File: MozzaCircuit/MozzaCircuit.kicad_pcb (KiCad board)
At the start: 2 copper layers, 11 parts

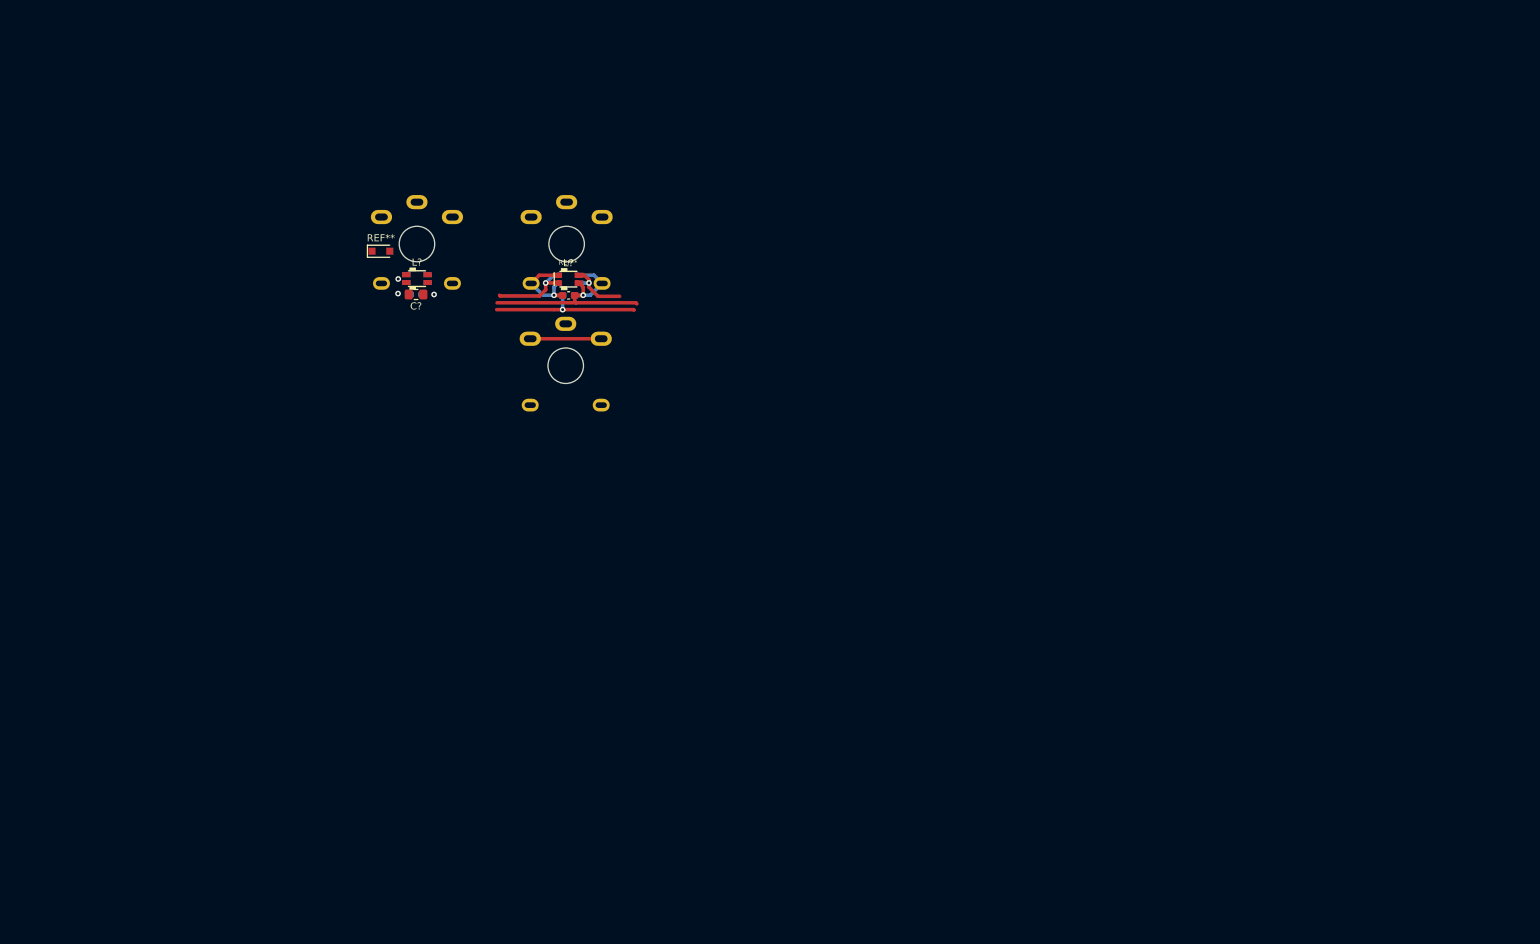
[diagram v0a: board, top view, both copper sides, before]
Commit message: init pcb
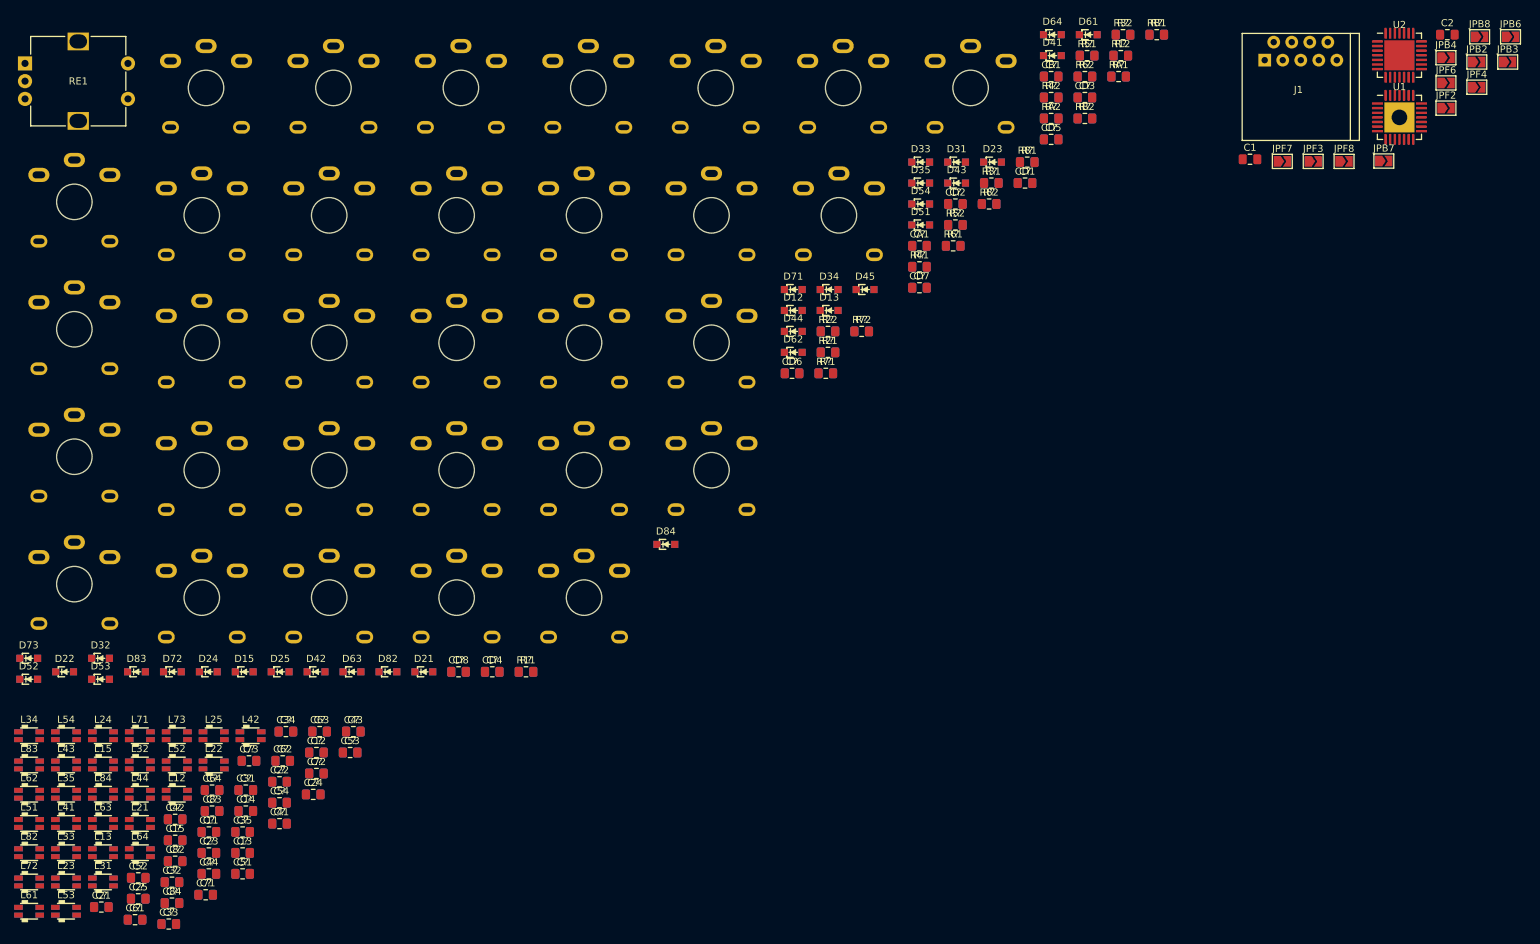
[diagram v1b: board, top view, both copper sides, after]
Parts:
- removed C?: C_2012, 00_KeyParts:C_2012
- removed L? (x2): WS2812B, 00_KeyParts:WS2812B_2020_rev
- removed REF** (x3): ChocV2_rev, 00_KeyParts:ChocV2_rev
- removed REF** (x3): C_0603_1608Metric_Pad1.08x0.95mm_HandSolder, Capacitor_SMD:C_0603_1608Metric_Pad1.08x0.95mm_HandSolder
- removed REF**: D_SOD-323_HandSoldering, Diode_SMD:D_SOD-323_HandSoldering
- removed REF**: WS2812C-2020, 00_KeyParts:LED_WS2812C-2020_BackMount_v2
- added C1: 0.1u, 00_KeyParts:C_2012, F.Cu at (206.2, 46.5)
- added C11: 0.1u, 00_KeyParts:C_2012_rev, F.Cu at (59.6, 141.2)
- added C12: C_Small, 00_KeyParts:C_2012_rev, F.Cu at (74.7, 130.1)
- added C13: C_Small, 00_KeyParts:C_2012_rev, F.Cu at (64.3, 144.2)
- added C14: C_Small, 00_KeyParts:C_2012_rev, F.Cu at (64.8, 138.3)
- added C15: C_Small, 00_KeyParts:C_2012_rev, F.Cu at (54.8, 142.4)
- added C2: C_Small, 00_KeyParts:C_2012, F.Cu at (234.0, 28.9)
- added C21: C_Small, 00_KeyParts:C_2012_rev, F.Cu at (44.4, 151.8)
- added C22: C_Small, 00_KeyParts:C_2012_rev, F.Cu at (69.5, 134.2)
- added C23: C_Small, 00_KeyParts:C_2012_rev, F.Cu at (59.6, 144.2)
- added C24: C_Small, 00_KeyParts:C_2012_rev, F.Cu at (74.3, 136.0)
- added C25: C_Small, 00_KeyParts:C_2012_rev, F.Cu at (49.6, 150.7)
- added C31: C_Small, 00_KeyParts:C_2012_rev, F.Cu at (64.8, 135.3)
- added C32: C_Small, 00_KeyParts:C_2012_rev, F.Cu at (54.4, 148.3)
- added C33: C_Small, 00_KeyParts:C_2012_rev, F.Cu at (53.9, 154.2)
- added C34: C_Small, 00_KeyParts:C_2012_rev, F.Cu at (70.4, 127.1)
- added C35: C_Small, 00_KeyParts:C_2012_rev, F.Cu at (64.3, 141.2)
- added C41: C_Small, 00_KeyParts:C_2012_rev, F.Cu at (69.5, 140.1)
- added C42: C_Small, 00_KeyParts:C_2012_rev, F.Cu at (54.8, 139.5)
- added C43: C_Small, 00_KeyParts:C_2012_rev, F.Cu at (79.9, 127.1)
- added C44: C_Small, 00_KeyParts:C_2012_rev, F.Cu at (59.6, 147.1)
- added C51: C_Small, 00_KeyParts:C_2012_rev, F.Cu at (64.3, 147.1)
- added C52: C_Small, 00_KeyParts:C_2012_rev, F.Cu at (49.6, 147.7)
- added C53: C_Small, 00_KeyParts:C_2012_rev, F.Cu at (79.5, 130.1)
- added C54: C_Small, 00_KeyParts:C_2012_rev, F.Cu at (69.5, 137.1)
- added C61: C_Small, 00_KeyParts:C_2012_rev, F.Cu at (49.2, 153.6)
- added C62: C_Small, 00_KeyParts:C_2012_rev, F.Cu at (70.0, 131.2)
- added C63: C_Small, 00_KeyParts:C_2012_rev, F.Cu at (75.2, 127.1)
- added C64: C_Small, 00_KeyParts:C_2012_rev, F.Cu at (60.0, 135.3)
- added C71: C_Small, 00_KeyParts:C_2012_rev, F.Cu at (59.1, 150.1)
- added C72: C_Small, 00_KeyParts:C_2012_rev, F.Cu at (74.7, 133.0)
- added C73: C_Small, 00_KeyParts:C_2012_rev, F.Cu at (65.2, 131.2)
- added C82: C_Small, 00_KeyParts:C_2012_rev, F.Cu at (54.8, 145.4)
- added C83: C_Small, 00_KeyParts:C_2012_rev, F.Cu at (60.0, 138.3)
- added C84: C_Small, 00_KeyParts:C_2012_rev, F.Cu at (54.4, 151.3)
- added CA1: 33n, 00_KeyParts:C_2012_rev, F.Cu at (159.7, 58.7)
- added CB1: C_Small, 00_KeyParts:C_2012_rev, F.Cu at (178.2, 34.8)
- added CD1: 33n, 00_KeyParts:C_2012_rev, F.Cu at (174.6, 49.8)
- added CD2: C_Small, 00_KeyParts:C_2012_rev, F.Cu at (164.7, 52.8)
- added CD3: C_Small, 00_KeyParts:C_2012_rev, F.Cu at (183.0, 37.8)
- added CD4: C_Small, 00_KeyParts:C_2012_rev, F.Cu at (99.5, 118.7)
- added CD5: C_Small, 00_KeyParts:C_2012_rev, F.Cu at (178.2, 43.7)
- added CD6: C_Small, 00_KeyParts:C_2012_rev, F.Cu at (141.7, 76.6)
- added CD7: C_Small, 00_KeyParts:C_2012_rev, F.Cu at (159.7, 64.6)
- added CD8: C_Small, 00_KeyParts:C_2012_rev, F.Cu at (94.8, 118.7)
- added D12: D_Small, 00_KeyParts:D_SOD-323_both_sides, F.Cu at (141.9, 67.8)
- added D13: D_Small, 00_KeyParts:D_SOD-323_both_sides, F.Cu at (147.0, 67.8)
- added D15: D_Small, 00_KeyParts:D_SOD-323_both_sides, F.Cu at (64.6, 118.7)
- added D21: D_Small, 00_KeyParts:D_SOD-323_both_sides, F.Cu at (89.9, 118.7)
- added D22: D_Small, 00_KeyParts:D_SOD-323_both_sides, F.Cu at (39.3, 118.7)
- added D23: D_Small, 00_KeyParts:D_SOD-323_both_sides, F.Cu at (170.0, 46.9)
- added D24: D_Small, 00_KeyParts:D_SOD-323_both_sides, F.Cu at (59.5, 118.7)
- added D25: D_Small, 00_KeyParts:D_SOD-323_both_sides, F.Cu at (69.6, 118.7)
- added D31: D_Small, 00_KeyParts:D_SOD-323_both_sides, F.Cu at (164.9, 46.9)
- added D32: D_Small, 00_KeyParts:D_SOD-323_both_sides, F.Cu at (44.3, 116.8)
- added D33: D_Small, 00_KeyParts:D_SOD-323_both_sides, F.Cu at (159.9, 46.9)
- added D34: D_Small, 00_KeyParts:D_SOD-323_both_sides, F.Cu at (147.0, 64.8)
- added D35: D_Small, 00_KeyParts:D_SOD-323_both_sides, F.Cu at (159.9, 49.8)
- added D41: D_Small, 00_KeyParts:D_SOD-323_both_sides, F.Cu at (178.4, 31.9)
- added D42: D_Small, 00_KeyParts:D_SOD-323_both_sides, F.Cu at (74.7, 118.7)
- added D43: D_Small, 00_KeyParts:D_SOD-323_both_sides, F.Cu at (164.9, 49.8)
- added D44: D_Small, 00_KeyParts:D_SOD-323_both_sides, F.Cu at (141.9, 70.7)
- added D45: D_Small, 00_KeyParts:D_SOD-323_both_sides, F.Cu at (152.0, 64.8)
- added D51: D_Small, 00_KeyParts:D_SOD-323_both_sides, F.Cu at (159.9, 55.7)
- added D52: D_Small, 00_KeyParts:D_SOD-323_both_sides, F.Cu at (34.2, 119.7)
- added D53: D_Small, 00_KeyParts:D_SOD-323_both_sides, F.Cu at (44.3, 119.7)
- added D54: D_Small, 00_KeyParts:D_SOD-323_both_sides, F.Cu at (159.9, 52.8)
- added D61: D_Small, 00_KeyParts:D_SOD-323_both_sides, F.Cu at (183.5, 28.9)
- added D62: D_Small, 00_KeyParts:D_SOD-323_both_sides, F.Cu at (141.9, 73.7)
- added D63: D_Small, 00_KeyParts:D_SOD-323_both_sides, F.Cu at (79.7, 118.7)
- added D64: D_Small, 00_KeyParts:D_SOD-323_both_sides, F.Cu at (178.4, 28.9)
- added D71: D_Small, 00_KeyParts:D_SOD-323_both_sides, F.Cu at (141.9, 64.8)
- added D72: D_Small, 00_KeyParts:D_SOD-323_both_sides, F.Cu at (54.4, 118.7)
- added D73: D_Small, 00_KeyParts:D_SOD-323_both_sides, F.Cu at (34.2, 116.8)
- added D82: D_Small, 00_KeyParts:D_SOD-323_both_sides, F.Cu at (84.8, 118.7)
- added D83: D_Small, 00_KeyParts:D_SOD-323_both_sides, F.Cu at (49.4, 118.7)
- added D84: D_Small, 00_KeyParts:D_SOD-323_both_sides, F.Cu at (124.0, 100.7)
- added J1: 8P8C_both_sides, 00_KeyParts:RJ45_Molex_0955032884_both_sides, F.Cu at (213.4, 30.0)
- added JPB2: SolderJumper_2_Open, Jumper:SolderJumper-2_P1.3mm_Open_TrianglePad1.0x1.5mm, F.Cu at (238.2, 32.8)
- added JPB3: SolderJumper_2_Open, Jumper:SolderJumper-2_P1.3mm_Open_TrianglePad1.0x1.5mm, F.Cu at (242.5, 32.8)
- added JPB4: SolderJumper_2_Open, Jumper:SolderJumper-2_P1.3mm_Open_TrianglePad1.0x1.5mm, F.Cu at (233.8, 32.2)
- added JPB6: SolderJumper_2_Open, Jumper:SolderJumper-2_P1.3mm_Open_TrianglePad1.0x1.5mm, F.Cu at (242.9, 29.2)
- added JPB7: SolderJumper_2_Open, Jumper:SolderJumper-2_P1.3mm_Open_TrianglePad1.0x1.5mm, F.Cu at (225.1, 46.7)
- added JPB8: SolderJumper_2_Open, Jumper:SolderJumper-2_P1.3mm_Open_TrianglePad1.0x1.5mm, F.Cu at (238.6, 29.2)
- added JPF2: SolderJumper_2_Open, Jumper:SolderJumper-2_P1.3mm_Open_TrianglePad1.0x1.5mm, F.Cu at (233.8, 39.3)
- added JPF3: SolderJumper_2_Open, Jumper:SolderJumper-2_P1.3mm_Open_TrianglePad1.0x1.5mm, F.Cu at (215.1, 46.8)
- added JPF4: SolderJumper_2_Open, Jumper:SolderJumper-2_P1.3mm_Open_TrianglePad1.0x1.5mm, F.Cu at (238.2, 36.3)
- added JPF6: SolderJumper_2_Open, Jumper:SolderJumper-2_P1.3mm_Open_TrianglePad1.0x1.5mm, F.Cu at (233.8, 35.7)
- added JPF7: SolderJumper_2_Open, Jumper:SolderJumper-2_P1.3mm_Open_TrianglePad1.0x1.5mm, F.Cu at (210.8, 46.8)
- added JPF8: SolderJumper_2_Open, Jumper:SolderJumper-2_P1.3mm_Open_TrianglePad1.0x1.5mm, F.Cu at (219.5, 46.8)
- added L12: WS2812-2020_both_sides, 00_KeyParts:WS2812B_2020_rev, F.Cu at (55.1, 135.9)
- added L13: WS2812-2020_both_sides, 00_KeyParts:WS2812B_2020_rev, F.Cu at (44.7, 144.2)
- added L15: WS2812-2020_both_sides, 00_KeyParts:WS2812B_2020_rev, F.Cu at (44.7, 131.8)
- added L21: WS2812-2020_both_sides, 00_KeyParts:WS2812B_2020_rev, F.Cu at (49.9, 140.0)
- added L22: WS2812-2020_both_sides, 00_KeyParts:WS2812B_2020_rev, F.Cu at (60.3, 131.8)
- added L23: WS2812-2020_both_sides, 00_KeyParts:WS2812B_2020_rev, F.Cu at (39.5, 148.3)
- added L24: WS2812-2020_both_sides, 00_KeyParts:WS2812B_2020_rev, F.Cu at (44.7, 127.7)
- added L25: WS2812-2020_both_sides, 00_KeyParts:WS2812B_2020_rev, F.Cu at (60.3, 127.7)
- added L31: WS2812-2020_both_sides, 00_KeyParts:WS2812B_2020_rev, F.Cu at (44.7, 148.3)
- added L32: WS2812-2020_both_sides, 00_KeyParts:WS2812B_2020_rev, F.Cu at (49.9, 131.8)
- added L33: WS2812-2020_both_sides, 00_KeyParts:WS2812B_2020_rev, F.Cu at (39.5, 144.2)
- added L34: WS2812-2020_both_sides, 00_KeyParts:WS2812B_2020_rev, F.Cu at (34.3, 127.7)
- added L35: WS2812-2020_both_sides, 00_KeyParts:WS2812B_2020_rev, F.Cu at (39.5, 135.9)
- added L41: WS2812-2020_both_sides, 00_KeyParts:WS2812B_2020_rev, F.Cu at (39.5, 140.0)
- added L42: WS2812-2020_both_sides, 00_KeyParts:WS2812B_2020_rev, F.Cu at (65.5, 127.7)
- added L43: WS2812-2020_both_sides, 00_KeyParts:WS2812B_2020_rev, F.Cu at (39.5, 131.8)
- added L44: WS2812-2020_both_sides, 00_KeyParts:WS2812B_2020_rev, F.Cu at (49.9, 135.9)
- added L51: WS2812-2020_both_sides, 00_KeyParts:WS2812B_2020_rev, F.Cu at (34.3, 140.0)
- added L52: WS2812-2020_both_sides, 00_KeyParts:WS2812B_2020_rev, F.Cu at (55.1, 131.8)
- added L53: WS2812-2020_both_sides, 00_KeyParts:WS2812B_2020_rev, F.Cu at (39.5, 152.4)
- added L54: WS2812-2020_both_sides, 00_KeyParts:WS2812B_2020_rev, F.Cu at (39.5, 127.7)
- added L61: WS2812-2020_both_sides, 00_KeyParts:WS2812B_2020_rev, F.Cu at (34.3, 152.4)
- added L62: WS2812-2020_both_sides, 00_KeyParts:WS2812B_2020_rev, F.Cu at (34.3, 135.9)
- added L63: WS2812-2020_both_sides, 00_KeyParts:WS2812B_2020_rev, F.Cu at (44.7, 140.0)
- added L64: WS2812-2020_both_sides, 00_KeyParts:WS2812B_2020_rev, F.Cu at (49.9, 144.2)
- added L71: WS2812-2020_both_sides, 00_KeyParts:WS2812B_2020_rev, F.Cu at (49.9, 127.7)
- added L72: WS2812-2020_both_sides, 00_KeyParts:WS2812B_2020_rev, F.Cu at (34.3, 148.3)
- added L73: WS2812-2020_both_sides, 00_KeyParts:WS2812B_2020_rev, F.Cu at (55.1, 127.7)
- added L82: WS2812-2020_both_sides, 00_KeyParts:WS2812B_2020_rev, F.Cu at (34.3, 144.2)
- added L83: WS2812-2020_both_sides, 00_KeyParts:WS2812B_2020_rev, F.Cu at (34.3, 131.8)
- added L84: WS2812-2020_both_sides, 00_KeyParts:WS2812B_2020_rev, F.Cu at (44.7, 135.9)
- added R11: 10k, 00_KeyParts:R_2012_rev, F.Cu at (104.3, 118.7)
- added R12: 4k7, 00_KeyParts:R_2012_rev, F.Cu at (188.0, 31.9)
- added R21: R_Small_US, 00_KeyParts:R_2012_rev, F.Cu at (146.8, 73.7)
- added R22: R_Small_US, 00_KeyParts:R_2012_rev, F.Cu at (146.8, 70.7)
- added R31: R_Small_US, 00_KeyParts:R_2012_rev, F.Cu at (169.8, 49.8)
- added R32: R_Small_US, 00_KeyParts:R_2012_rev, F.Cu at (188.4, 28.9)
- added R41: R_Small_US, 00_KeyParts:R_2012_rev, F.Cu at (159.7, 61.6)
- added R42: R_Small_US, 00_KeyParts:R_2012_rev, F.Cu at (178.2, 37.8)
- added R51: R_Small_US, 00_KeyParts:R_2012_rev, F.Cu at (183.3, 31.9)
- added R52: R_Small_US, 00_KeyParts:R_2012_rev, F.Cu at (164.7, 55.7)
- added R61: R_Small_US, 00_KeyParts:R_2012_rev, F.Cu at (164.4, 58.7)
- added R62: R_Small_US, 00_KeyParts:R_2012_rev, F.Cu at (183.0, 34.8)
- added R71: R_Small_US, 00_KeyParts:R_2012_rev, F.Cu at (146.5, 76.6)
- added R72: R_Small_US, 00_KeyParts:R_2012_rev, F.Cu at (151.5, 70.7)
- added R81: R_Small_US, 00_KeyParts:R_2012_rev, F.Cu at (174.9, 46.9)
- added R82: R_Small_US, 00_KeyParts:R_2012_rev, F.Cu at (169.5, 52.8)
- added RA1: 10k, 00_KeyParts:R_2012_rev, F.Cu at (187.7, 34.8)
- added RA2: 4k7, 00_KeyParts:R_2012_rev, F.Cu at (178.2, 40.7)
- added RB1: R_Small_US, 00_KeyParts:R_2012_rev, F.Cu at (193.1, 28.9)
- added RB2: R_Small_US, 00_KeyParts:R_2012_rev, F.Cu at (183.0, 40.7)
- added RE1: RotaryEncoder_Switch, 00_KeyParts:RotaryEncoder_Bourns_PEC12R-4215F, F.Cu at (41.2, 35.5)
- added SW12: SW_ChocV2_rev, 00_KeyParts:ChocV2_rev, F.Cu at (113.0, 36.4)
- added SW13: SW_ChocV2_rev, 00_KeyParts:ChocV2_rev, F.Cu at (76.5, 108.2)
- added SW15: SW_ChocV2_rev, 00_KeyParts:ChocV2_rev, F.Cu at (40.6, 106.3)
- added SW21: SW_ChocV2_rev, 00_KeyParts:ChocV2_rev, F.Cu at (58.6, 72.3)
- added SW22: SW_ChocV2_rev, 00_KeyParts:ChocV2_rev, F.Cu at (59.2, 36.4)
- added SW23: SW_ChocV2_rev, 00_KeyParts:ChocV2_rev, F.Cu at (130.4, 72.3)
- added SW24: SW_ChocV2_rev, 00_KeyParts:ChocV2_rev, F.Cu at (40.6, 52.5)
- added SW25: SW_ChocV2_rev, 00_KeyParts:ChocV2_rev, F.Cu at (77.1, 36.4)
- added SW31: SW_ChocV2_rev, 00_KeyParts:ChocV2_rev, F.Cu at (148.9, 36.4)
- added SW32: SW_ChocV2_rev, 00_KeyParts:ChocV2_rev, F.Cu at (112.4, 72.3)
- added SW33: SW_ChocV2_rev, 00_KeyParts:ChocV2_rev, F.Cu at (76.5, 90.3)
- added SW34: SW_ChocV2_rev, 00_KeyParts:ChocV2_rev, F.Cu at (112.4, 54.4)
- added SW35: SW_ChocV2_rev, 00_KeyParts:ChocV2_rev, F.Cu at (94.5, 72.3)
- added SW41: SW_ChocV2_rev, 00_KeyParts:ChocV2_rev, F.Cu at (166.9, 36.4)
- added SW42: SW_ChocV2_rev, 00_KeyParts:ChocV2_rev, F.Cu at (40.6, 70.4)
- added SW43: SW_ChocV2_rev, 00_KeyParts:ChocV2_rev, F.Cu at (130.4, 90.3)
- added SW44: SW_ChocV2_rev, 00_KeyParts:ChocV2_rev, F.Cu at (94.5, 90.3)
- added SW51: SW_ChocV2_rev, 00_KeyParts:ChocV2_rev, F.Cu at (76.5, 54.4)
- added SW52: SW_ChocV2_rev, 00_KeyParts:ChocV2_rev, F.Cu at (131.0, 36.4)
- added SW53: SW_ChocV2_rev, 00_KeyParts:ChocV2_rev, F.Cu at (130.4, 54.4)
- added SW54: SW_ChocV2_rev, 00_KeyParts:ChocV2_rev, F.Cu at (94.5, 54.4)
- added SW61: SW_ChocV2_rev, 00_KeyParts:ChocV2_rev, F.Cu at (58.6, 108.2)
- added SW62: SW_ChocV2_rev, 00_KeyParts:ChocV2_rev, F.Cu at (76.5, 72.3)
- added SW63: SW_ChocV2_rev, 00_KeyParts:ChocV2_rev, F.Cu at (94.5, 108.2)
- added SW64: SW_ChocV2_rev, 00_KeyParts:ChocV2_rev, F.Cu at (58.6, 90.3)
- added SW71: SW_ChocV2_rev, 00_KeyParts:ChocV2_rev, F.Cu at (95.1, 36.4)
- added SW72: SW_ChocV2_rev, 00_KeyParts:ChocV2_rev, F.Cu at (40.6, 88.4)
- added SW73: SW_ChocV2_rev, 00_KeyParts:ChocV2_rev, F.Cu at (148.3, 54.4)
- added SW82: SW_ChocV2_rev, 00_KeyParts:ChocV2_rev, F.Cu at (58.6, 54.4)
- added SW83: SW_ChocV2_rev, 00_KeyParts:ChocV2_rev, F.Cu at (112.4, 90.3)
- added SW84: SW_ChocV2_rev, 00_KeyParts:ChocV2_rev, F.Cu at (112.4, 108.2)
- added U1: MCP23017_ML, 00_KeyParts:QFN-28-1EP_6x6mm_P0.65mm_EP4.25x4.25mm_Hand, F.Cu at (227.3, 40.6)
- added U2: MCP23017_ML, 00_KeyParts:QFN-28-1EP_6x6mm_P0.65mm_EP4.25x4.25mm_Hand_NoTP, F.Cu at (227.3, 31.8)
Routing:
- net (no net): track 96.9 -> 0.00 mm, vias 8 -> 0
